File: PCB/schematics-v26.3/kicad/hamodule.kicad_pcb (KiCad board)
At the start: 4 copper layers, 131.9 x 84 mm, 206 parts, among them J1 GND|5V, J10 Tx|Rx, J11 Sda|Scl, J12 3|9, J13 13|12, J14 3.3v|GND|7|15, J15 2604-1104, J16 2604-1104, J17 TestPoint, J19 TestPoint, J2 2604-1102, J3 USB_C_Receptacle_USB2.0, J4 GND|3.3V, J5 Jumper 3.3v, J6 2604-1104, J7 2604-1104, J8 5v|GND|Do, J9 Screen, K1 AQG22205, K2 AQG22205, K3 AQG22205, K4 AQG22205, K5 AQG22205, K6 AQG22205, K7 AQG22205, K8 AQG22205, SW1 USB | PS, SW2 Reset, SW3 Boot, U1 LD1117AV33, U10 SN74LV1T34DBV, U11 ULN2803A, U12 TCAL6416, U14 74AHC1G04, U2 USBLC6-2SC6, U3 ESP32-S3-WROOM-2, U4 LDA210, U5 LDA210, U6 LDA210, U7 LDA210, U8 SHT4x, U9 SN74LVCH8T245

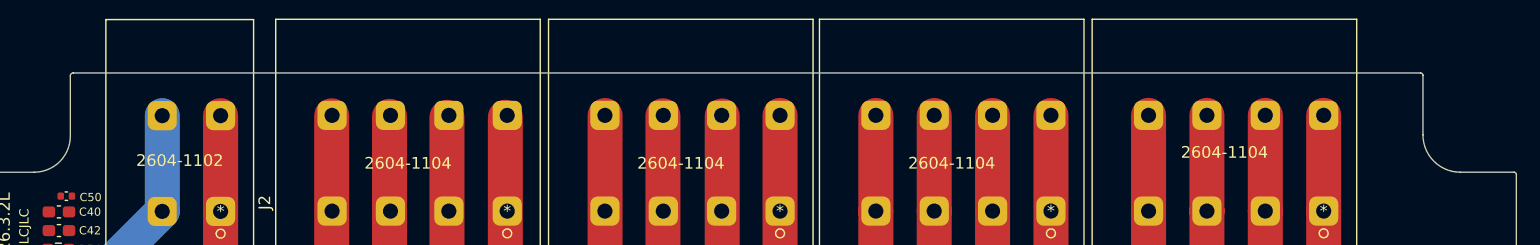
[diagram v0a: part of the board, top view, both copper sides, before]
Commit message: Version 26.3
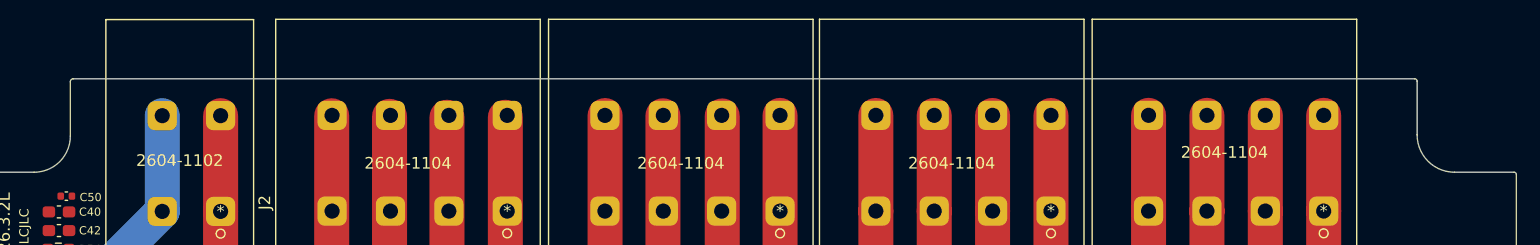
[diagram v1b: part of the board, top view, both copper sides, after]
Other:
- board size 131.9 x 84 mm -> 131.9 x 83.5 mm
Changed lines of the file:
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@@
 	)
 	(gr_line
-		(start 146.8 31.5)
-		(end 31.391411 31.5)
+		(start 146.3 32)
+		(end 31.391411 32)
 		(stroke
 			(width 0.05)
@@
 	)
 	(gr_arc
-		(start 146.8 31.5)
-		(mid 146.941421 31.558579)
-		(end 147 31.7)
+		(start 146.3 32)
+		(mid 146.441421 32.058579)
+		(end 146.5 32.2)
 		(stroke
 			(width 0.05)
@@
 	)
 	(gr_arc
-		(start 150.2 40)
-		(mid 147.937258 39.062742)
-		(end 147 36.8)
+		(start 149.7 40)
+		(mid 147.437258 39.062742)
+		(end 146.5 36.8)
 		(stroke
 			(width 0.05)
@@
 	(gr_line
 		(start 31.15 36.9)
-		(end 31.15 31.7414)
+		(end 31.15 32.241411)
 		(stroke
 			(width 0.05)
@@
 	)
 	(gr_line
-		(start 150.2 40)
+		(start 149.7 40)
 		(end 154.8 40)
 		(stroke
@@
 	)
 	(gr_line
-		(start 147 36.8)
-		(end 147 31.7)
+		(start 146.5 36.8)
+		(end 146.5 32.2)
 		(stroke
 			(width 0.05)
@@
 	)
 	(gr_arc
-		(start 31.15 31.741411)
-		(mid 31.220708 31.570708)
-		(end 31.391411 31.5)
+		(start 31.15 32.241411)
+		(mid 31.220708 32.070708)
+		(end 31.391411 32)
 		(stroke
 			(width 0.05)
@@
 		(layer "Dwgs.User")
 		(pts
-			(xy 31.6 115.5) (xy 31.45 31.03)
+			(xy 31.6 115.5) (xy 31.391411 32)
 		)
 		(height -17.498728)
@@
 			(keep_text_aligned yes)
 		)
-		(gr_text "84.4701 mm"
-			(at 15.176298 73.294032 -89.8982555)
+		(gr_text "83.5003 mm"
+			(at 15.147028 73.79084 -89.85687064)
 			(layer "Dwgs.User")
 			(effects
@@
 		(layer "Dwgs.User")
 		(pts
-			(xy 146.55 31.5) (xy 146.55 40.03)
+			(xy 146.549551 32.006668) (xy 146.55 40.03)
 		)
 		(height -10.5)
@@
 			(keep_text_aligned yes)
 		)
-		(gr_text "8.5300 mm"
-			(at 155.899975 35.764992 90)
+		(gr_text "8.0233 mm"
+			(at 155.899731 36.017779 270.0032135)
 			(layer "Dwgs.User")
 			(effects
@@
 		(layer "Dwgs.User")
 		(pts
-			(xy 31.129289 32.4) (xy 147 32.399544)
+			(xy 31.129289 32.4) (xy 146.5 32.398891)
 		)
 		(height -8)
@@
 			(keep_text_aligned yes)
 		)
-		(gr_text "115.8707 mm"
-			(at 88.798318 23.449757 0.0002254829975)
+		(gr_text "115.3707 mm"
+			(at 88.549384 23.449394 0.0005512518225)
 			(layer "Dwgs.User")
 			(effects
@@
 		(layer "Dwgs.User")
 		(pts
-			(xy 147 36.8) (xy 155.05 36.83)
+			(xy 146.5 36.8) (xy 155.05 36.83)
 		)
 		(height -12.460317)
@@
 			(keep_text_aligned yes)
 		)
-		(gr_text "8.0501 mm"
-			(at 151.075722 23.204778 359.7864763)
+		(gr_text "8.5501 mm"
+			(at 150.822755 23.204767 359.798963)
 			(layer "Dwgs.User")
 			(effects
